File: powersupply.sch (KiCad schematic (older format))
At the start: 0 parts

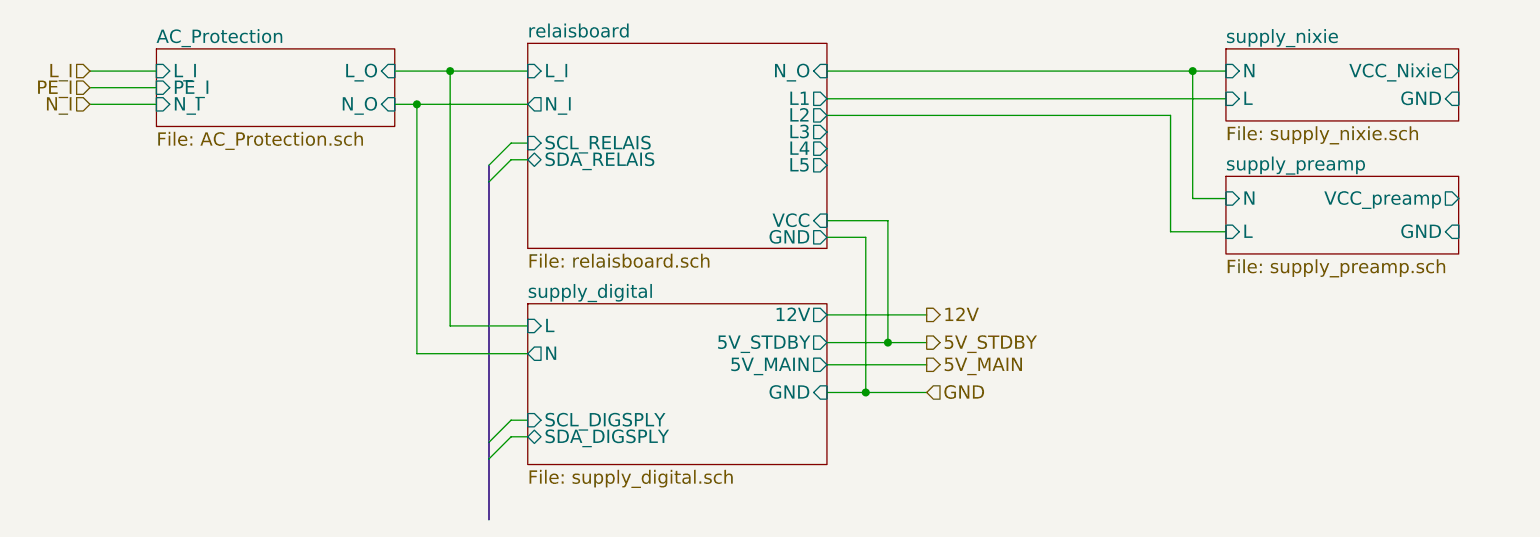
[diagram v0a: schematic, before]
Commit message: blub
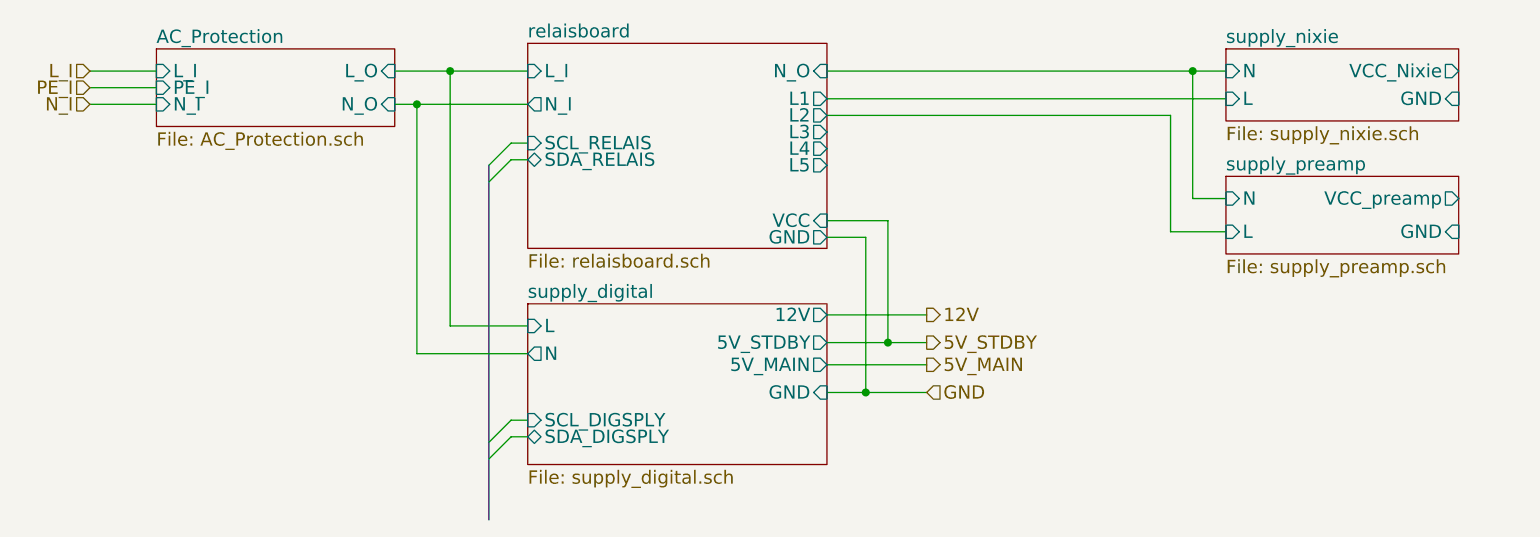
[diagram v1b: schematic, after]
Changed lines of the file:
@@
 $Descr A3 16535 11693
 encoding utf-8
-Sheet 4 12
+Sheet 4 13
 Title ""
 Date ""
@@
 $EndSheet
 Wire Wire Line
-	3125 1625 3375 1625
+	3125 1625 3725 1625
 Wire Wire Line
-	3375 1625 3725 1625
-Wire Wire Line
-	3125 1775 3225 1775
-Wire Wire Line
-	3225 1775 3725 1775
+	3125 1775 3725 1775
 Wire Wire Line
 	3725 2775 3375 2775
@@
 	3725 2025 3650 2025
 Wire Bus Line
-	3550 2050 3550 2125
-Wire Bus Line
-	3550 2125 3550 3300
-Wire Bus Line
-	3550 3300 3550 3375
-Wire Bus Line
-	3550 3375 3550 3650
+	3550 2050 3550 3650
 Entry Wire Line
 	3550 3300 3650 3200
@@
 GND
 Wire Wire Line
-	5075 2850 5350 2850
-Wire Wire Line
-	5350 2850 5525 2850
+	5075 2850 5525 2850
 Wire Wire Line
 	5525 2950 5075 2950
 Wire Wire Line
-	5075 3075 5250 3075
-Wire Wire Line
-	5250 3075 5525 3075
+	5075 3075 5525 3075
 Wire Wire Line
 	5075 2375 5250 2375
@@
 $EndSheet
 Wire Wire Line
-	5075 1625 6725 1625
-Wire Wire Line
-	6725 1625 6875 1625
+	5075 1625 6875 1625
 Wire Wire Line
 	5075 1750 6875 1750

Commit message: daily commit
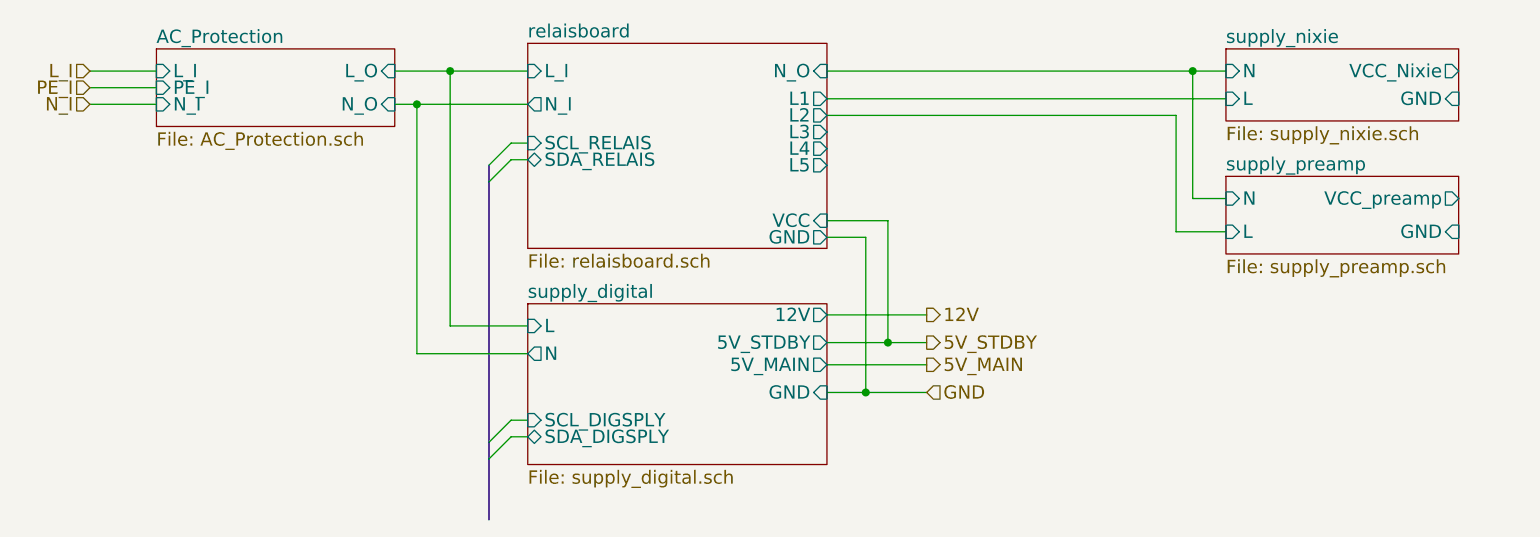
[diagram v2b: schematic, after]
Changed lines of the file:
@@
 $EndSheet
 Wire Wire Line
-	3125 1625 3725 1625
+	3125 1625 3375 1625
 Wire Wire Line
-	3125 1775 3725 1775
+	3375 1625 3725 1625
+Wire Wire Line
+	3125 1775 3225 1775
+Wire Wire Line
+	3225 1775 3725 1775
 Wire Wire Line
 	3725 2775 3375 2775
@@
 	3725 2025 3650 2025
 Wire Bus Line
-	3550 2050 3550 3650
+	3550 2050 3550 2125
+Wire Bus Line
+	3550 2125 3550 3300
+Wire Bus Line
+	3550 3300 3550 3375
+Wire Bus Line
+	3550 3375 3550 3650
 Entry Wire Line
 	3550 3300 3650 3200
@@
 GND
 Wire Wire Line
-	5075 2850 5525 2850
+	5075 2850 5350 2850
+Wire Wire Line
+	5350 2850 5525 2850
 Wire Wire Line
 	5525 2950 5075 2950
 Wire Wire Line
-	5075 3075 5525 3075
+	5075 3075 5250 3075
+Wire Wire Line
+	5250 3075 5525 3075
 Wire Wire Line
 	5075 2375 5250 2375
@@
 $EndSheet
 Wire Wire Line
-	5075 1625 6875 1625
+	5075 1625 6725 1625
+Wire Wire Line
+	6725 1625 6875 1625
 Wire Wire Line
 	5075 1750 6875 1750
@@
 Connection ~ 6725 1625
 Wire Wire Line
-	5075 1825 6625 1825
+	5075 1825 6650 1825
 Wire Wire Line
-	6625 1825 6625 2350
+	6650 1825 6650 2350
 Wire Wire Line
-	6625 2350 6875 2350
+	6650 2350 6875 2350
 $EndSCHEMATC
